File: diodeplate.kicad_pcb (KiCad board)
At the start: 2 copper layers, 160 x 160 mm, 85 parts, among them SW1 TS-1185EC-C-D-B, SW2 TS-1185EC-C-D-B, SW3 TS-1185EC-C-D-B, U1 ESP32-WROOM-32E, U2 CP2102-GMR, U3 U262-161N-4BVC11, U4 BL1117-33CX, U5 UMH3N, U6 SN74AHCT32QPWRQ1

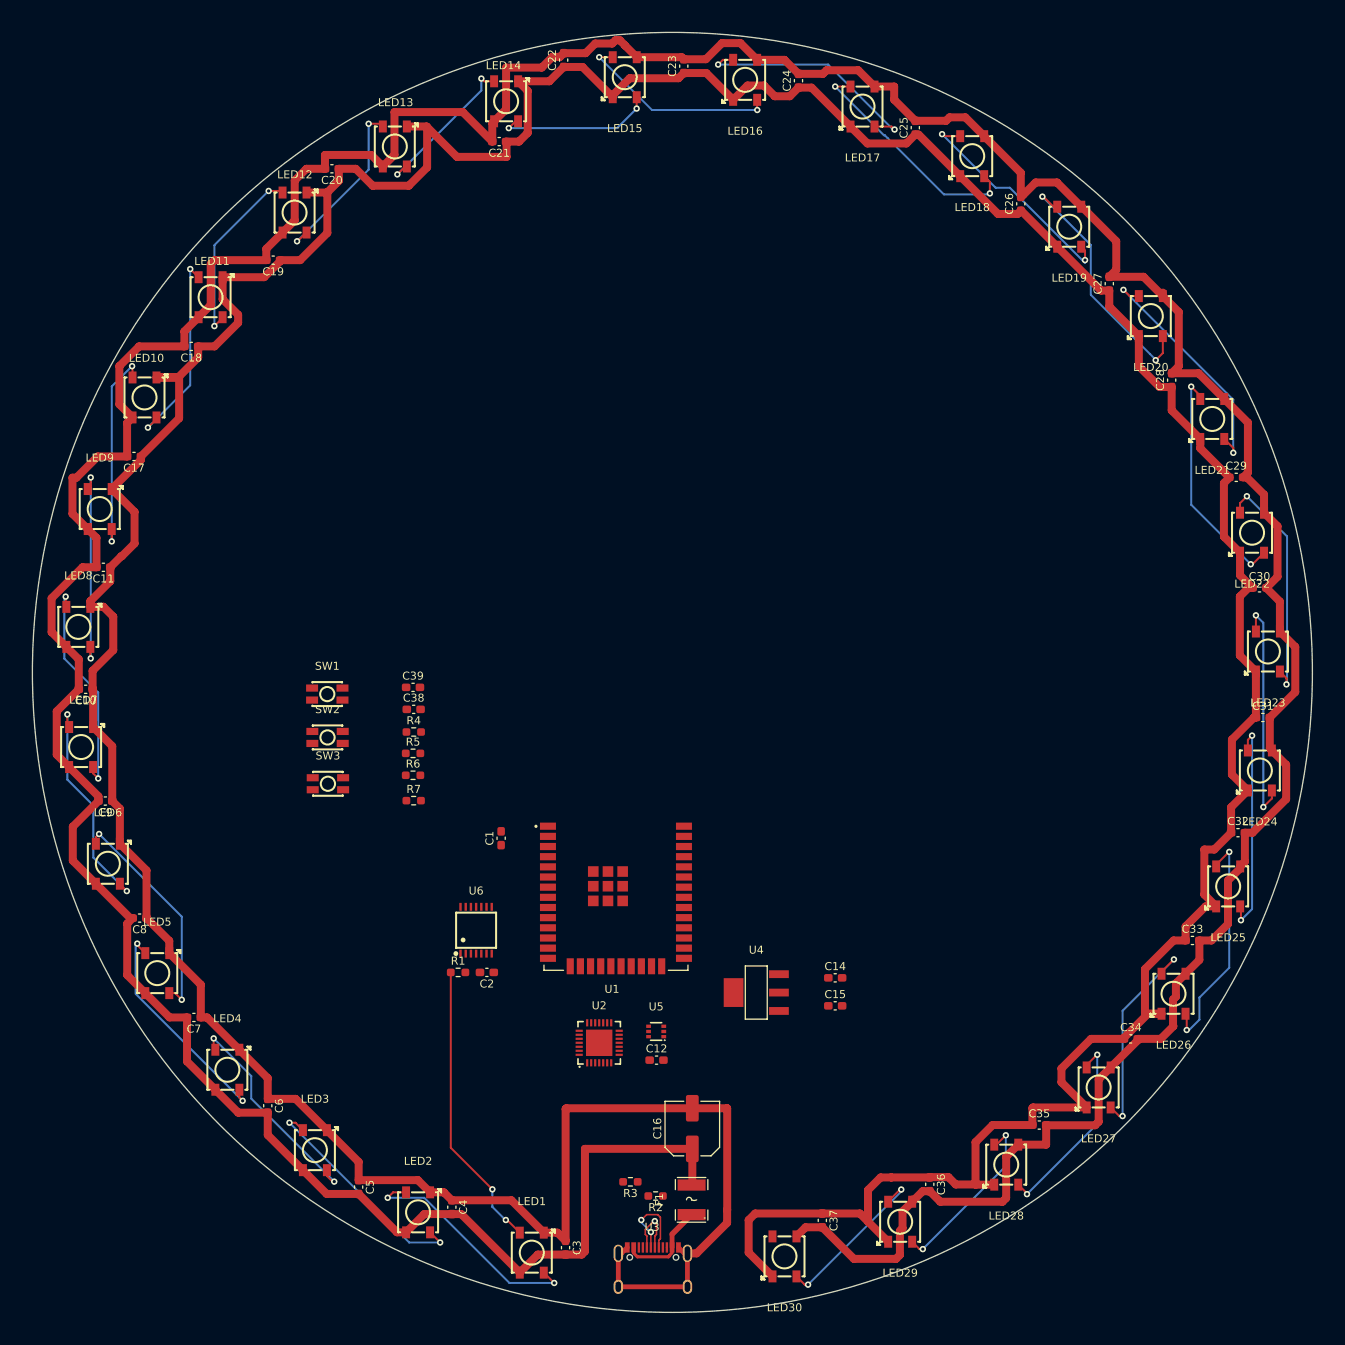
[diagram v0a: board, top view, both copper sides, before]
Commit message: add jlcpscb folder
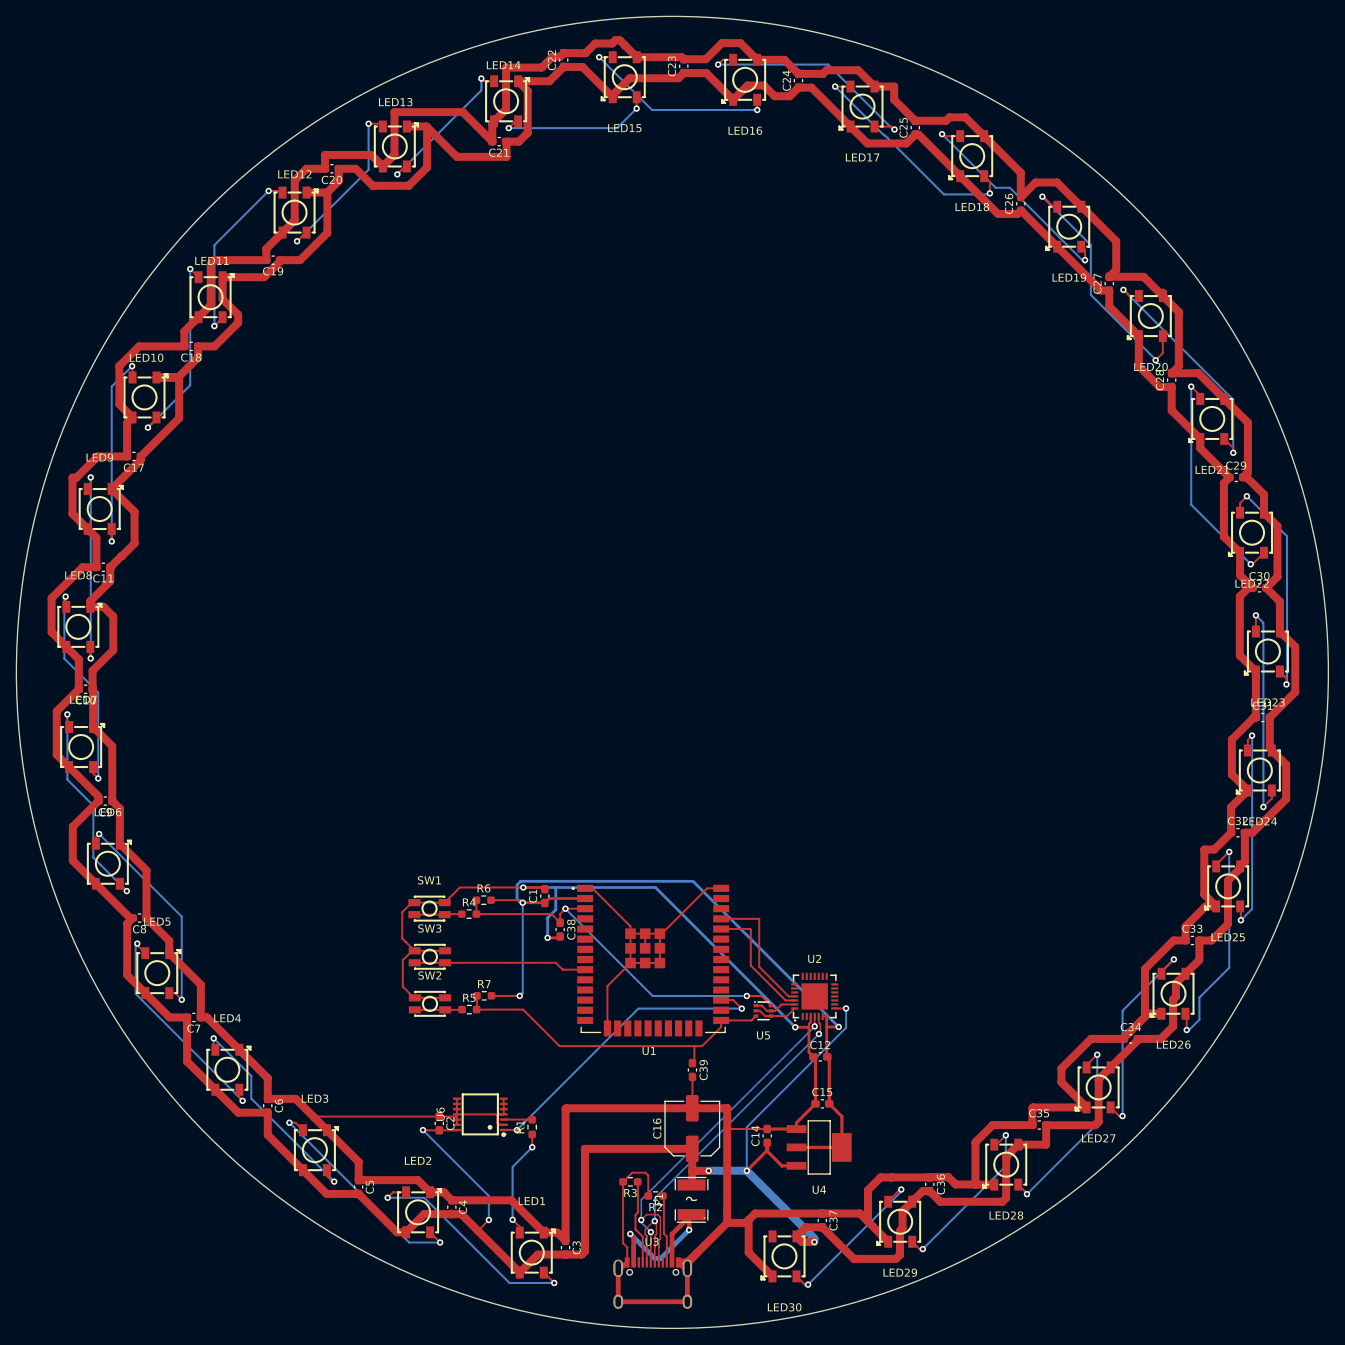
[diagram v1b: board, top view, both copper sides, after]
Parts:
- moved C39 59.2 mm to (219.1, 192.3), turned to -90 degrees
- moved SW2 35.7 mm to (186.3, 184.1)
- moved C38 33.1 mm to (202.6, 174.8), turned to -90 degrees
- moved R5 32.8 mm to (191.2, 184.8)
- moved SW1 29.7 mm to (186.2, 172.2)
- moved U2 27.6 mm to (234.4, 183.1)
- moved R7 25.9 mm to (193.1, 183.1)
- moved SW3 25.1 mm to (186.3, 178.2)
- moved R4 23.8 mm to (191.2, 172.8)
- moved U6 23.0 mm to (192.6, 197.9), turned to 90 degrees
- moved C14 21.5 mm to (228.4, 200.6), turned to 90 degrees
- moved R1 21.4 mm to (199.1, 199.5), turned to 90 degrees
- moved U4 20.9 mm to (234.9, 202.0), turned to 180 degrees
- moved C12 20.5 mm to (235.1, 190.7)
- moved C2 19.8 mm to (187.5, 199.0), turned to -90 degrees
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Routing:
- net GND: track 626.0 -> 844.1 mm, vias 0 -> 3
- net +3V3: track 0.00 -> 102.9 mm, vias 0 -> 3
- net +5V: track 585.5 -> 665.0 mm, vias 0 -> 6
- net RESET: track 0.00 -> 47.9 mm, vias 0 -> 2
- net IO0: track 0.00 -> 42.8 mm
- net IO16/LED1: track 0.00 -> 39.1 mm, vias 0 -> 2
- net USB-C DATA +: track 10.6 -> 49.2 mm, vias 2 -> 3
- net USB-C DATA -: track 7.41 -> 45.6 mm, vias 1 -> 2
- net LED DATA OUT: track 36.4 -> 13.7 mm
- net IO33/MAINBUTTON: track 0.00 -> 21.7 mm
- net TXD: track 0.00 -> 16.7 mm
- net RXD: track 0.00 -> 15.5 mm
- net USB-C CC1: track 0.00 -> 10.6 mm
- net VBUS: track 11.7 -> 21.5 mm, vias 0 -> 2
- net USB-C CC2: track 0.03 -> 8.53 mm
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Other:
- board size 160 x 160 mm -> 164 x 164 mm
